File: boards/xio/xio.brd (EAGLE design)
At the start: 170 x 100 mm, 146 parts, among them Y2 NX3225SA-12.000MHZ-STD-CSR-1

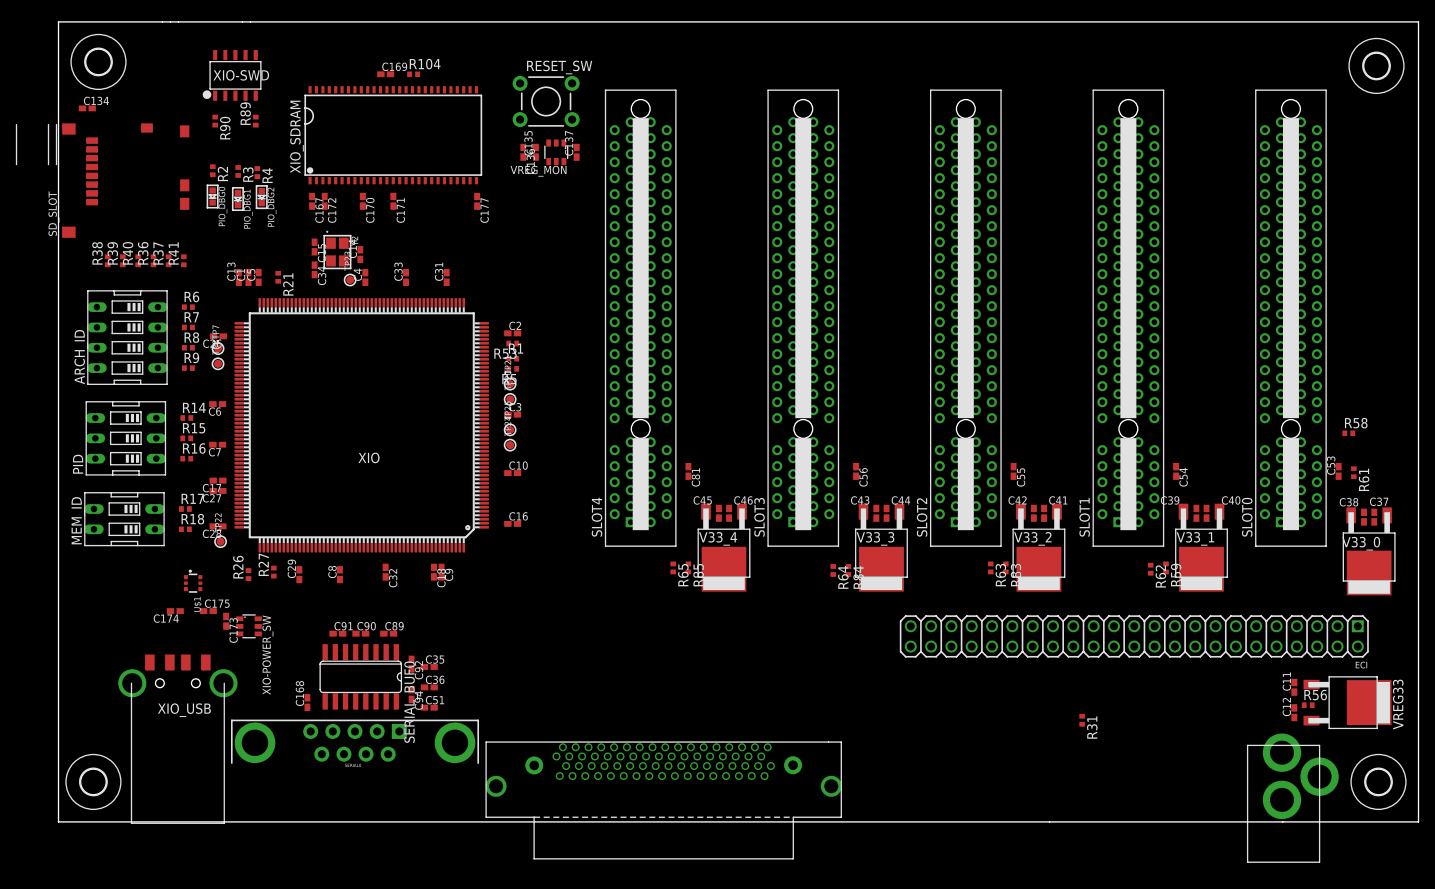
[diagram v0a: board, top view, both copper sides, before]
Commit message: Latest snapshot
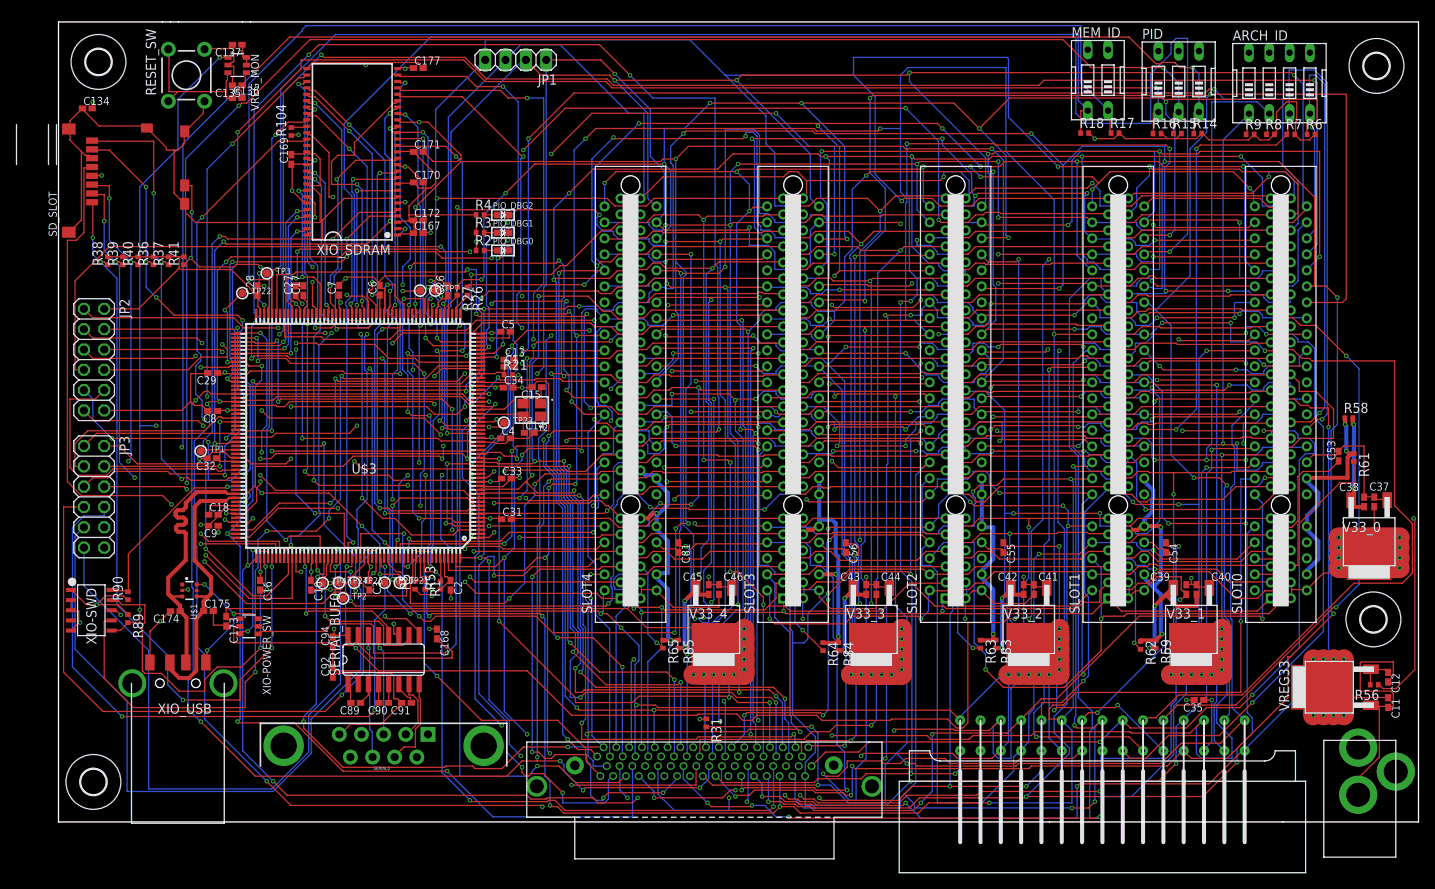
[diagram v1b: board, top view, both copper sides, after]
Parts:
- removed C36, C51: 0.1uF, rcl:C0402K
- removed ECI: eci, microbuilder:2X23
- removed XIO: STM32H753B-XIO, sjg-stm32:PQFP208
- added JP1: (no value), pinhead:1X04
- added JP2, JP3: (no value), pinhead:2X06
- added TP1, TP2, TP3, TP4: (no value), microbuilder:TESTPOINT_ROUND_1MM
- added U$2: A8_CART, sjg-con:A8_CART
- added U$3: XIO, sjg-stm32:PQFP208
- moved ARCH_ID 147.5 mm to (152.6, 92.3), turned to 0 degrees
- moved R6 142.0 mm to (156.6, 85.9)
- moved R7 139.9 mm to (154.0, 85.9)
- moved PID 139.0 mm to (140.0, 92.5), turned to 0 degrees
- moved R8 137.9 mm to (151.5, 85.9)
- moved R9 135.9 mm to (149.0, 85.9)
- moved MEM_ID 133.5 mm to (129.9, 92.7), turned to 0 degrees
- moved R14 131.3 mm to (142.4, 86.0)
- moved R15 129.6 mm to (139.9, 86.0)
- moved R16 127.9 mm to (137.3, 86.0)
- moved R17 125.3 mm to (132.1, 86.1)
- moved R18 122.8 mm to (128.3, 86.1)
- moved C35 96.3 mm to (142.6, 15.2), turned to 180 degrees
- moved XIO-SWD 69.2 mm to (4.11, 26.5), turned to 270 degrees
- moved R89 64.2 mm to (8.68, 25.4), turned to 270 degrees
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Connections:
- removed net I2C_SCL: SLOT0.B42, SLOT1.B42, SLOT2.B42, SLOT3.B42, SLOT4.B42, XIO.91
- removed net I2C_SDA: SLOT0.B43, SLOT1.B43, SLOT2.B43, SLOT3.B43, SLOT4.B43, XIO.90
- new net AUX_CTS: JP1.1, SLOT0.B46, SLOT1.B46, SLOT2.B46, SLOT3.B46, SLOT4.B46, U$3.30
- new net AUX_RTS: JP1.4, SLOT0.B47, SLOT1.B47, SLOT2.B47, SLOT3.B47, SLOT4.B47, U$3.29
- new net AUX_RX: JP1.2, SLOT0.B48, SLOT1.B48, SLOT2.B48, SLOT3.B48, SLOT4.B48, U$3.27
- new net AUX_TX: JP1.3, SLOT0.B49, SLOT1.B49, SLOT2.B49, SLOT3.B49, SLOT4.B49, U$3.28
- new net N$3: TP1.P$1, U$3.134
- new net N$4: TP2.P$1, U$3.178
- new net N$5: TP3.P$1, U$3.102
- new net N$6: TP4.P$1, U$3.175
- new net USRA_CLK: JP2.1, U$3.45
- new net USRA_D0: JP2.3, U$3.35
- new net USRA_D1: JP2.4, U$3.36
- new net USRA_D2: JP2.5, U$3.37
- new net USRA_D3: JP2.6, U$3.38
- new net USRA_D4: JP2.7, U$3.57
- new net USRA_D5: JP2.8, U$3.58
- new net USRA_D6: JP2.9, U$3.138
- new net USRA_D7: JP2.10, U$3.139
- new net USRA_MISC: JP2.11, U$3.10
- new net USRB_CLK: JP3.1, U$3.130
- new net USRB_D0: JP3.3, U$3.126
- new net USRB_D1: JP3.4, U$3.127
- new net USRB_D2: JP3.5, U$3.128
- new net USRB_D3: JP3.6, U$3.186
- new net USRB_D4: JP3.7, U$3.187
- new net USRB_D5: JP3.8, U$3.188
- new net USRB_D6: JP3.9, U$3.189
- new net USRB_D7: JP3.10, U$3.190
- new net USRB_MISC: JP3.11, U$3.177
- net !RESET!: now also U$3.34; no longer XIO.34
- net !VHDCI_EXSEL!: now also U$3.68; no longer ECI.1, XIO.68
- net !VHDCI_IRQ!: now also U$3.69; no longer ECI.2, XIO.69
- net !VHDCI_MPD!: now also U$3.67; no longer ECI.3, XIO.67
- net +3V3: now also JP2.2, JP3.2, U$3.103, U$3.115, U$3.124, U$3.137, U$3.15, U$3.150, U$3.158, U$3.171, U$3.185, U$3.204, U$3.26, U$3.39, U$3.52, U$3.59, U$3.6, U$3.73, U$3.83, U$3.94; no longer XIO.103, XIO.115, XIO.124, XIO.137, XIO.15, XIO.150, XIO.158, XIO.171, XIO.185, XIO.204, XIO.26, XIO.39, XIO.52, XIO.59, XIO.6, XIO.73, XIO.83, XIO.94
- net +5V: now also U$2.P13; no longer C36.1, C51.1, ECI.42, ECI.44, ECI.46
- net ARCH0: now also U$3.96
- net ARCH1: now also U$3.97
- net ARCH2: now also U$3.98
- net ARCH3: now also U$3.99
- net A_OK: now also U$3.176
- net GND: now also JP2.12, JP3.12, U$2.PB, U$3.114, U$3.125, U$3.136, U$3.14, U$3.149, U$3.170, U$3.184, U$3.202, U$3.25, U$3.40, U$3.51, U$3.60, U$3.72, U$3.82, U$3.93; no longer C36.2, C51.2, ECI.41, ECI.43, ECI.45, SLOT0.B41, SLOT0.B44, SLOT1.B41, SLOT1.B44, SLOT2.B41, SLOT2.B44, SLOT3.B41, SLOT3.B44, SLOT4.B41, SLOT4.B44, XIO.114, XIO.125, XIO.136, XIO.14, XIO.149, XIO.170, XIO.184, XIO.202, XIO.25, XIO.40, XIO.51, XIO.60, XIO.72, XIO.82, XIO.93
- net MEM0: now also U$3.100
- net MEM1: now also U$3.101
- net N$1: now also U$3.33; no longer XIO.33
- net N$107: now also U$3.9; no longer XIO.192
- net N$108: now also U$3.111; no longer XIO.193
- net N$109: now also U$3.112; no longer XIO.104
- net N$11: now also U$3.197; no longer XIO.197
- net N$110: now also U$3.113; no longer XIO.31
- net N$111: now also U$3.31; no longer XIO.179
- net N$112: now also U$3.133; no longer XIO.180
- net N$13: now also U$3.46; no longer XIO.169
- net N$14: now also U$3.47; no longer XIO.172
- net N$15: now also U$3.48; no longer XIO.173
- net N$2: now also U$3.32; no longer XIO.32
- net N$34: now also U$3.167; no longer XIO.43
- net N$35: now also U$3.172; no longer XIO.50
- net N$39: now also U$3.169; no longer XIO.45
- net N$40: now also U$3.168; no longer XIO.44
- net N$57: now also U$3.54; no longer XIO.105
- net N$61: now also U$3.56; no longer XIO.107
- net N$64: now also U$3.160; no longer XIO.160
- net N$65: now also U$3.53; no longer XIO.199
- net N$7: now also U$3.203; no longer XIO.203
- net N$86: now also U$3.50; no longer XIO.61
- net N$93: now also U$3.8; no longer XIO.63
- net PID0: now also U$3.151
- net PID1: now also U$3.152
- net PID2: now also U$3.153
- net SD0: now also U$3.140
- net SD1: now also U$3.141
- net SD2: now also U$3.161
- net SD3: now also U$3.162
- net SDCD: now also U$3.173
- net SDCLK: now also U$3.163
- net SDCMD: now also U$3.166
- net SPI_CLK: now also SLOT0.B41, SLOT1.B41, SLOT2.B41, SLOT3.B41, SLOT4.B41; no longer SLOT0.B45, SLOT1.B45, SLOT2.B45, SLOT3.B45, SLOT4.B45
- net SPI_IRQ0: now also SLOT0.B42, U$3.179; no longer SLOT0.B48, XIO.99
- net SPI_IRQ1: now also SLOT1.B42, U$3.180; no longer SLOT1.B48, XIO.100
- net SPI_IRQ2: now also SLOT2.B42, U$3.181; no longer SLOT2.B48, XIO.101
- net SPI_IRQ3: now also SLOT3.B42, U$3.182; no longer SLOT3.B48, XIO.102
- net SPI_IRQ4: now also SLOT4.B42, U$3.183; no longer SLOT4.B48
- net SPI_MISO: now also SLOT0.B43, SLOT1.B43, SLOT2.B43, SLOT3.B43, SLOT4.B43, U$3.55; no longer SLOT0.B46, SLOT1.B46, SLOT2.B46, SLOT3.B46, SLOT4.B46, XIO.106
- net SPI_MOSI: now also SLOT0.B44, SLOT1.B44, SLOT2.B44, SLOT3.B44, SLOT4.B44; no longer SLOT0.B47, SLOT1.B47, SLOT2.B47, SLOT3.B47, SLOT4.B47
- net SPI_SS0: now also SLOT0.B45, U$3.1; no longer SLOT0.B49, XIO.46
- net SPI_SS1: now also SLOT1.B45, U$3.2; no longer SLOT1.B49, XIO.47
- net SPI_SS2: now also SLOT2.B45, U$3.3; no longer SLOT2.B49, XIO.48
- net SPI_SS3: now also SLOT3.B45, U$3.4; no longer SLOT3.B49, XIO.130
- net SPI_SS4: now also SLOT4.B45, U$3.5; no longer SLOT4.B49, XIO.96
- net VHDCI_A0: now also U$2.P5, U$3.107; no longer ECI.5, XIO.35
- net VHDCI_A1: now also U$2.P4, U$3.106; no longer ECI.6, XIO.36
- net VHDCI_A10: now also U$2.PP, U$3.194; no longer ECI.15, XIO.161
- net VHDCI_A11: now also U$2.PN, U$3.193; no longer ECI.16, XIO.162
- net VHDCI_A12: now also U$2.PK, U$3.192; no longer ECI.17, XIO.163
- net VHDCI_A13: now also U$3.63; no longer ECI.18, XIO.8
- net VHDCI_A14: now also U$3.62; no longer ECI.19, XIO.9
- net VHDCI_A15: now also U$3.61; no longer ECI.20, XIO.10
- net VHDCI_A2: now also U$2.P3, U$3.105; no longer ECI.7, XIO.37
- net VHDCI_A3: now also U$2.P2, U$3.104; no longer ECI.8, XIO.38
- net VHDCI_A4: now also U$2.PC, U$3.91; no longer ECI.9, XIO.57
- net VHDCI_A5: now also U$2.PD, U$3.90; no longer ECI.10, XIO.58
- net VHDCI_A6: now also U$2.PE, U$3.199; no longer ECI.11, XIO.138
- net VHDCI_A7: now also U$2.PF, U$3.198; no longer ECI.12, XIO.139
- net VHDCI_A8: now also U$2.PH, U$3.196; no longer ECI.13, XIO.140
- net VHDCI_A9: now also U$2.PJ, U$3.195; no longer ECI.14, XIO.141
- net VHDCI_AUDIO_SIO: no longer ECI.4
- net VHDCI_CCTL: now also U$2.P15, U$3.95; no longer ECI.21, XIO.95
- net VHDCI_CLK: now also U$2.PS, U$3.65; no longer ECI.22, XIO.65
- net VHDCI_D0: now also U$2.P10, U$3.154; no longer ECI.24, XIO.154
- net VHDCI_D1: now also U$2.P9, U$3.155; no longer ECI.25, XIO.155
- net VHDCI_D1XX: now also U$3.121; no longer ECI.23, XIO.121
- net VHDCI_D2: now also U$2.P8, U$3.156; no longer ECI.26, XIO.156
- net VHDCI_D3: now also U$2.PL, U$3.157; no longer ECI.27, XIO.157
- net VHDCI_D4: now also U$2.P6, U$3.205; no longer ECI.28, XIO.205
- net VHDCI_D5: now also U$2.P7, U$3.206; no longer ECI.29, XIO.206
- net VHDCI_D6: now also U$2.P11, U$3.207; no longer ECI.30, XIO.207
- net VHDCI_D7: now also U$2.PM, U$3.208; no longer ECI.31, XIO.208
- net VHDCI_GND: no longer ECI.32
- net VHDCI_HALT: now also U$3.123; no longer ECI.33, XIO.123
- net VHDCI_RD4: now also U$2.PA, U$3.66; no longer ECI.34, XIO.66
- net VHDCI_RD5: now also U$2.P14, U$3.64; no longer ECI.35, XIO.64
- net VHDCI_REF: now also U$3.120; no longer ECI.36, XIO.120
- net VHDCI_RSRVD0: now also U$3.7; no longer XIO.7
- net VHDCI_RSRVD1: now also U$3.11; no longer XIO.11
- net VHDCI_RSRVD2: now also U$3.12; no longer XIO.12
- net VHDCI_RSRVD3: now also U$3.13; no longer XIO.13
- net VHDCI_RSRVD4: now also U$3.19; no longer XIO.19
- net VHDCI_RSRVD5: now also U$3.20; no longer XIO.20
- net VHDCI_RSRVD6: now also U$3.21; no longer XIO.21
- net VHDCI_RST: now also U$3.122; no longer ECI.37, XIO.122
- net VHDCI_RW: now also U$2.PR, U$3.174; no longer ECI.38, XIO.174
- net VHDCI_S4: now also U$2.P1, U$3.119; no longer ECI.39, XIO.119
- net VHDCI_S5: now also U$2.P12, U$3.118; no longer ECI.40, XIO.118
- net XIO_RAM_A0: now also U$3.16; no longer XIO.16
- net XIO_RAM_A1: now also U$3.17; no longer XIO.17
- net XIO_RAM_A10: now also U$3.77; no longer XIO.77
- net XIO_RAM_A11: now also U$3.78; no longer XIO.78
- net XIO_RAM_A12: now also U$3.129; no longer XIO.129
- net XIO_RAM_A2: now also U$3.18; no longer XIO.18
- net XIO_RAM_A3: now also U$3.22; no longer XIO.22
- net XIO_RAM_A4: now also U$3.23; no longer XIO.23
- net XIO_RAM_A5: now also U$3.24; no longer XIO.24
- net XIO_RAM_A6: now also U$3.71; no longer XIO.71
- net XIO_RAM_A7: now also U$3.74; no longer XIO.74
- net XIO_RAM_A8: now also U$3.75; no longer XIO.75
- net XIO_RAM_A9: now also U$3.76; no longer XIO.76
- net XIO_RAM_BA0: now also U$3.131; no longer XIO.131
- net XIO_RAM_BA1: now also U$3.132; no longer XIO.132
- net XIO_RAM_CAS: now also U$3.191; no longer XIO.191
- net XIO_RAM_CLK: now also U$3.135; no longer XIO.135
- net XIO_RAM_D0: now also U$3.116; no longer XIO.116
- net XIO_RAM_D1: now also U$3.117; no longer XIO.117
- net XIO_RAM_D10: now also U$3.87; no longer XIO.87
- net XIO_RAM_D11: now also U$3.88; no longer XIO.88
- net XIO_RAM_D12: now also U$3.89; no longer XIO.89
- net XIO_RAM_D13: now also U$3.108; no longer XIO.108
- net XIO_RAM_D14: now also U$3.109; no longer XIO.109
- net XIO_RAM_D15: now also U$3.110; no longer XIO.110
- net XIO_RAM_D2: now also U$3.164; no longer XIO.164
- net XIO_RAM_D3: now also U$3.165; no longer XIO.165
- net XIO_RAM_D4: now also U$3.79; no longer XIO.79
- net XIO_RAM_D5: now also U$3.80; no longer XIO.80
- net XIO_RAM_D6: now also U$3.81; no longer XIO.81
- net XIO_RAM_D7: now also U$3.84; no longer XIO.84
- net XIO_RAM_D8: now also U$3.85; no longer XIO.85
- net XIO_RAM_D9: now also U$3.86; no longer XIO.86
- net XIO_RAM_DQMH: now also U$3.201; no longer XIO.201
- net XIO_RAM_DQML: now also U$3.200; no longer XIO.200
- net XIO_RAM_RAS: now also U$3.70; no longer XIO.70
- net XIO_RAM_WE: now also U$3.49; no longer XIO.49
- net XIO_RX: now also U$3.44; no longer XIO.196
- net XIO_SWDCLK: now also U$3.159; no longer XIO.159
- net XIO_SWDIO: now also U$3.147; no longer XIO.147
- net XIO_TX: now also U$3.43; no longer XIO.195
- net XIO_USB_N: now also U$3.145; no longer XIO.145
- net XIO_USB_P: now also U$3.146; no longer XIO.146
- net XIO_VCAP1: now also U$3.92; no longer XIO.92
- net XIO_VCAP2: now also U$3.148; no longer XIO.148
- net XIO_VDDA: now also U$3.41, U$3.42; no longer XIO.41, XIO.42
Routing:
- net GND: track 0.00 -> 467.5 mm, vias 0 -> 33
- net VHDCI_RW: track 0.00 -> 402.0 mm, vias 0 -> 13
- net VHDCI_S5: track 0.00 -> 388.4 mm, vias 0 -> 13
- net +5V: track 0.00 -> 369.2 mm, vias 0 -> 64
- net VHDCI_D4: track 0.00 -> 342.4 mm, vias 0 -> 10
- net VHDCI_D3: track 0.00 -> 331.5 mm, vias 0 -> 5
- net VHDCI_RD5: track 0.00 -> 325.1 mm, vias 0 -> 8
- net VHDCI_REF: track 0.00 -> 315.5 mm, vias 0 -> 12
- net ARCH2: track 0.00 -> 311.7 mm, vias 0 -> 8
- net VHDCI_D1: track 0.00 -> 309.7 mm, vias 0 -> 7
- net VHDCI_A7: track 0.00 -> 296.4 mm, vias 0 -> 11
- net VHDCI_S4: track 0.00 -> 294.4 mm, vias 0 -> 10
- net VHDCI_CLK: track 0.00 -> 290.0 mm, vias 0 -> 11
- net VHDCI_D0: track 0.00 -> 287.8 mm, vias 0 -> 8
- net VHDCI_D2: track 0.00 -> 287.3 mm, vias 0 -> 9
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- added copper zone on layer 15, net +3V3
- added copper zone on layer 15, net +5V
- added copper zone on layer 2, net GND
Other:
- board text added: "Indent SD card slot Make parts for STM32F Neaten everything up Add 5v plane rectangle Add GND plane Add 3.3v plane"
- board text removed: "Indent SD card slot Make parts for STM32F Neaten everything up Make cartridge part 5650118-1 and place Add 5v plane rectangle Add GND plane Add 3.3v plane Find better (larger) USB ESD part"
